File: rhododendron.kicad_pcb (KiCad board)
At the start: 2 copper layers, 70.7 x 53.3 mm, 46 parts, among them J1 Conn_02x20_Odd_Even, J2 Conn_02x20_Odd_Even, J7 BONUS_ROW, U1 USB3343, Y1 26MHz

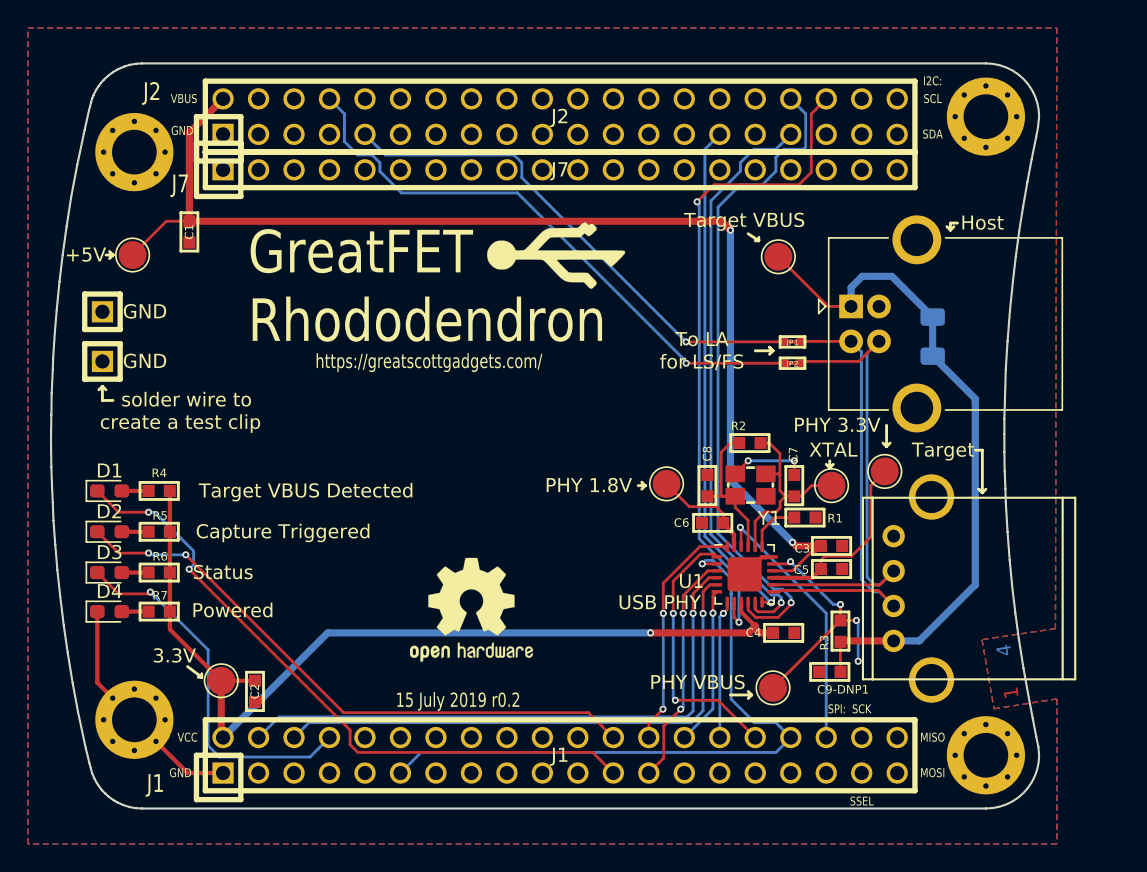
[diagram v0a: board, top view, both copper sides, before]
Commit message: r0.3: route the changes made in the r0.3 schematic
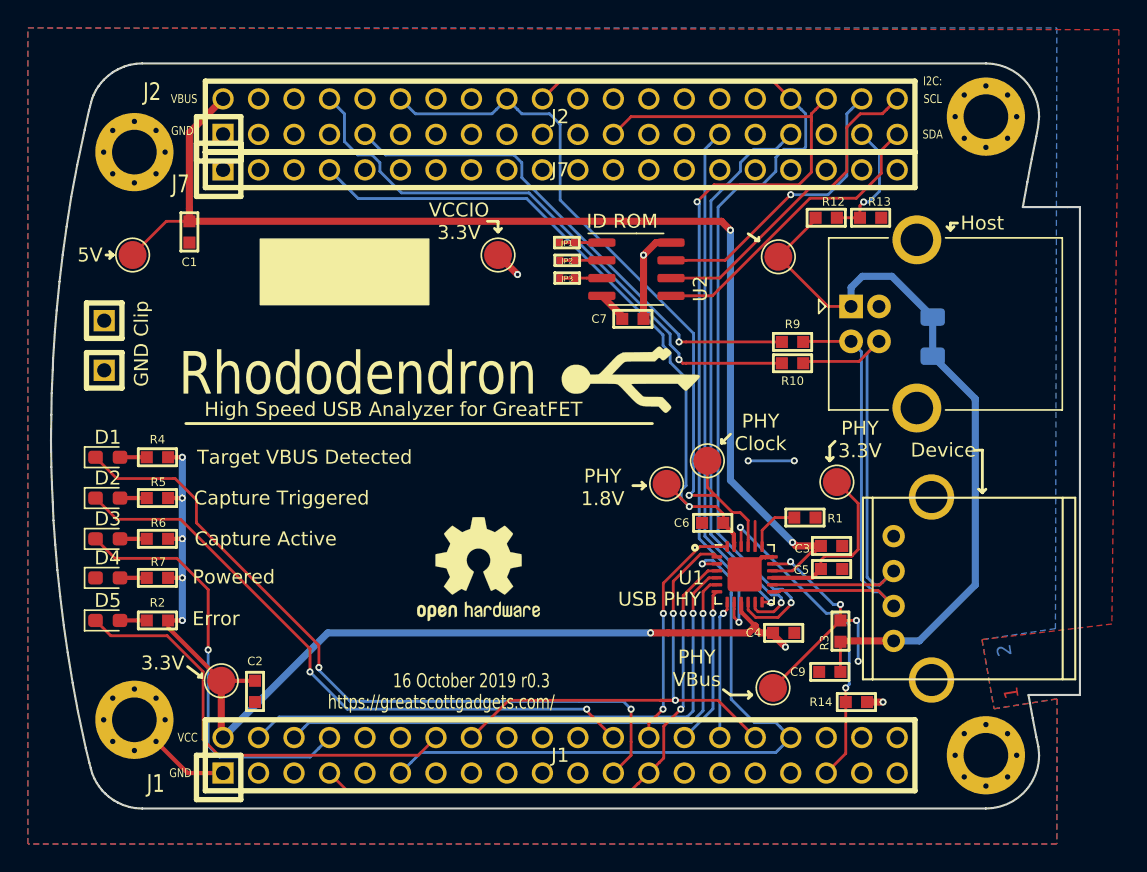
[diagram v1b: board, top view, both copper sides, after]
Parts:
- removed C8: 8.2pF, gsg-modules:0603
- removed PHY VBUS: TestPoint, TestPoint:TestPoint_Pad_D2.0mm
- removed XTAL: TestPoint, TestPoint:TestPoint_Pad_D2.0mm
- removed Y1: 26MHz, gsg-modules:XTAL3.2x2.5mm
- added D5: LED, LED_SMD:LED_0603_1608Metric_Pad1.05x0.95mm_HandSolder, F.Cu at (113.7, 108.5)
- added JP3: Jumper_NC_Small, gsg-modules:0402-SHORT-10MIL, F.Cu at (146.6, 83.9)
- added R10: 1K, gsg-modules:0603, F.Cu at (162.7, 90.0)
- added R12: 1K, gsg-modules:0603, F.Cu at (165.1, 79.6)
- added R13: 1K5, gsg-modules:0603, F.Cu at (168.3, 79.6)
- added R14: 10K, gsg-modules:0603, F.Cu at (167.3, 114.3)
- added R9: 1K, gsg-modules:0603, F.Cu at (162.7, 88.5)
- added TP4: TestPoint, TestPoint:TestPoint_Pad_D2.0mm, F.Cu at (156.6, 97.0)
- added TP6: TestPoint, TestPoint:TestPoint_Pad_D2.0mm, F.Cu at (161.3, 113.3)
- added TP7: TestPoint, TestPoint:TestPoint_Pad_D2.0mm, F.Cu at (141.6, 82.3)
- added U2: M24C02-FMN, Package_SO:SOIC-8_3.9x4.9mm_P1.27mm, F.Cu at (151.5, 83.3)
- C7: value 8.2pF -> 10nF
- R2: value 1M -> 330
- TP1: renamed from PHY 3.3V
- TP5: renamed from PHY 1.8V
- TP8: renamed from Target VBUS
- moved R2 44.3 mm to (117.2, 108.5), turned to 0 degrees
- moved JP2 17.7 mm to (146.6, 82.7)
- moved JP1 17.7 mm to (146.5, 81.4)
- moved C7 16.6 mm to (151.3, 86.9), turned to 0 degrees
- moved G*** 10.4 mm to (151.1, 91.2)
- moved TP1 3.51 mm to (165.9, 98.6)
- moved REF** 2.96 mm to (140.2, 104.8)
- moved D2 2.42 mm to (113.7, 99.7)
- moved R5 2.42 mm to (117.2, 99.7)
- moved D1 2.42 mm to (113.7, 96.8)
- moved D3 2.42 mm to (113.7, 102.6)
- moved D4 2.42 mm to (113.7, 105.4)
- moved R4 2.42 mm to (117.2, 96.8)
- moved R6 2.42 mm to (117.2, 102.6)
- moved R7 2.42 mm to (117.2, 105.4)
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- renumbered C9-DNP1 to C9, Target to Device, +5V to TP2, 3.3V to TP3, GND to TP9
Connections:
- net /LED_STATUS renamed /LED_CAPTURING
- C7 pad 2: /PHY_XO -> +3V3
- J1 pad 11: /ULPI_CLK -> +3V3
- J1 pad 14: /P5_2 -> /LED_ERROR
- J1 pad 16: /P1_6 -> /ULPI_DIR
- J1 pad 34: /ULPI_CLK -> +3V3
- J1 pad 35: /P2_0 -> /~PHY_RESET
- J1 pad 36: /~PHY_RESET -> /P6_3
- J1 pad 7: /P1_0 -> /ULPI_NXT
- J2 pad 12: /CLK2 -> /REFCLK
- J2 pad 18: /P2_5 -> /REFCLK
- J2 pad 20: /P2_3 -> /ULPI_DATA5
- J2 pad 23: /P7_2 -> /ULPI_DATA4
- J2 pad 37: /P3_5 -> /TARGET_VBUS_DETECT
- J2 pad 38: /P3_6 -> /I2C_EEPROM_WC
- J7 pad 10: GND -> /RTCX1
- J7 pad 20: VCC -> +3V3
- J7 pad 4: /ADC0_5 -> /PHY_VDD18
- JP1 pad 1: /LA_USB_D- -> GND
- JP1 pad 2: /USB_D- -> Net-(JP1-Pad2)
- JP2 pad 1: /LA_USB_D+ -> GND
- JP2 pad 2: /USB_D+ -> Net-(JP2-Pad2)
- R2 pad 1: /PHY_XO -> Net-(D5-Pad2)
- R2 pad 2: /PHY_XI -> +3V3
- U1 pad 2: /ULPI_CLK -> +3V3
- U1 pad 20: /PHY_XO -> Net-(U1-Pad20)
- U1 pad 21: /PHY_XI -> /REFCLK
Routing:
- net +3V3: track 66.8 -> 132.2 mm, vias 1 -> 11
- net /REFCLK: track 0.00 -> 53.3 mm, vias 0 -> 1
- net /ULPI_CLK: track 46.9 -> 0.00 mm, vias 1 -> 0
- net /PHY_VDD18: track 7.61 -> 49.7 mm, vias 0 -> 1
- net /LED_ERROR: track 0.00 -> 31.7 mm
- net /ULPI_NXT: track 16.9 -> 40.8 mm
- net /I2C0_SCL: track 0.00 -> 23.4 mm
- net /I2C0_SDA: track 0.00 -> 21.9 mm
- net /I2C_EEPROM_WC: track 0.00 -> 21.0 mm, vias 0 -> 1
- net /ULPI_DATA5: track 47.8 -> 66.7 mm
- net /ULPI_DIR: track 19.4 -> 36.2 mm
- net /ULPI_DATA4: track 47.8 -> 62.8 mm
- net /PHY_XO: track 14.6 -> 0.00 mm
- net /PHY_XI: track 11.6 -> 0.00 mm
- net GND: track 25.8 -> 16.0 mm
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- added copper zone on B.Cu, net +3V3
- removed copper zone on B.Cu, net VCC
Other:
- board size 70.7 x 53.3 mm -> 73.7 x 53.3 mm
- board text added: "16 October 2019 r0.3"
- board text added: "2"
- board text added: "3.3V"
- board text added: "5V"
- board text added: "Capture Active"
- board text added: "Error"
- board text added: "GND Clip"
- board text added: "High Speed USB Analyzer for GreatFET"
- board text added: "ID ROM"
- board text added: "PHY 1.8V"
- board text added: "PHY 3.3V"
- board text added: "PHY Clock"
- board text added: "PHY VBus"
- board text added: "Rhododendron"
- board text added: "VCCIO 3.3V"
- board text added: "design by Kate Temkin (@ktemkin); with help from Mikaela Szekely (@Qyriad)"
- board text removed: "15 July 2019 r0.2"
- board text removed: "4"
- board text removed: "GreatFET Rhododendron"
- board text removed: "MISO"
- board text removed: "MOSI"
- board text removed: "SCK"
- board text removed: "SPI:"
- board text removed: "SSEL"
- board text removed: "Status"
- board text removed: "To LA for LS/FS"
- board text removed: "design by @ktemkin; with help from @Qyriad"
- board text removed: "solder wire to create a test clip"
